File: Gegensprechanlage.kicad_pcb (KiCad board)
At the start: 2 copper layers, 42.4 x 27.8 mm, 13 parts, among them J1 To other, P1 22k, SW1 SW_Push, U1 LM386

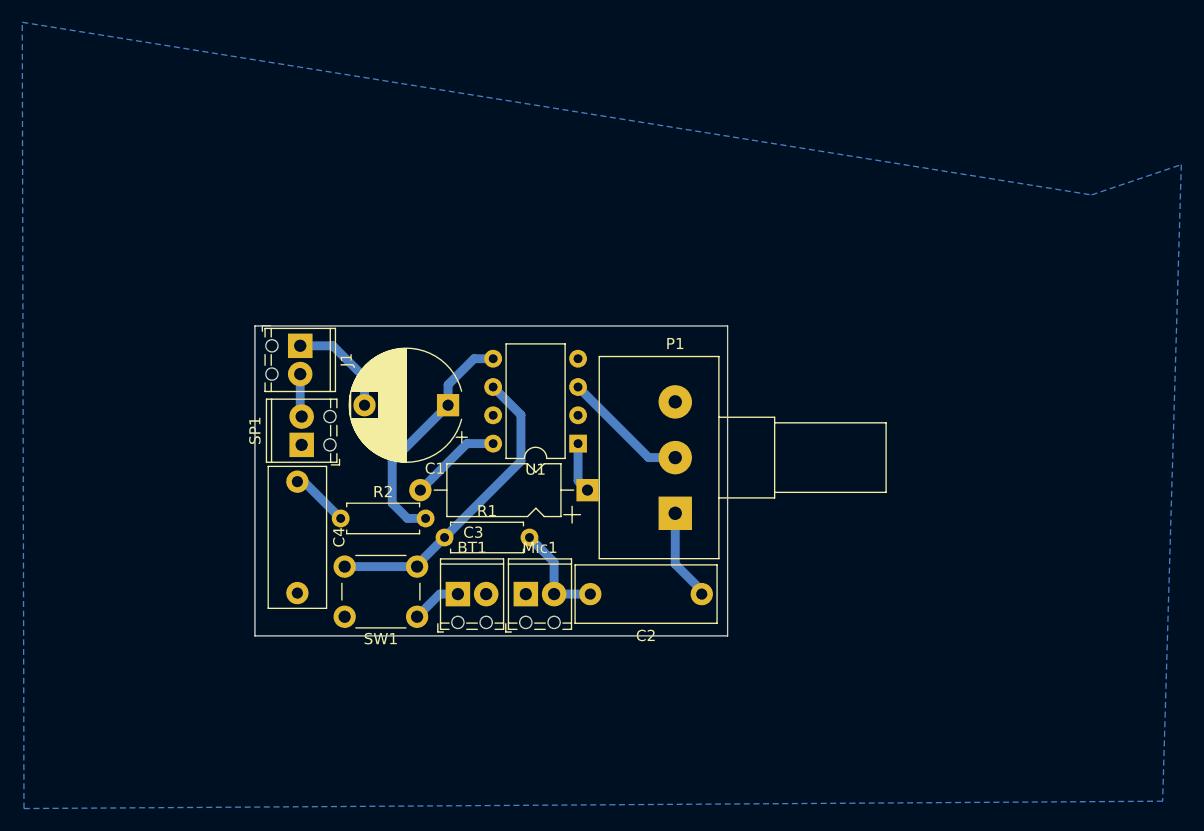
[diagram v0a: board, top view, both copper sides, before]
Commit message: Prepare for milling v1.0
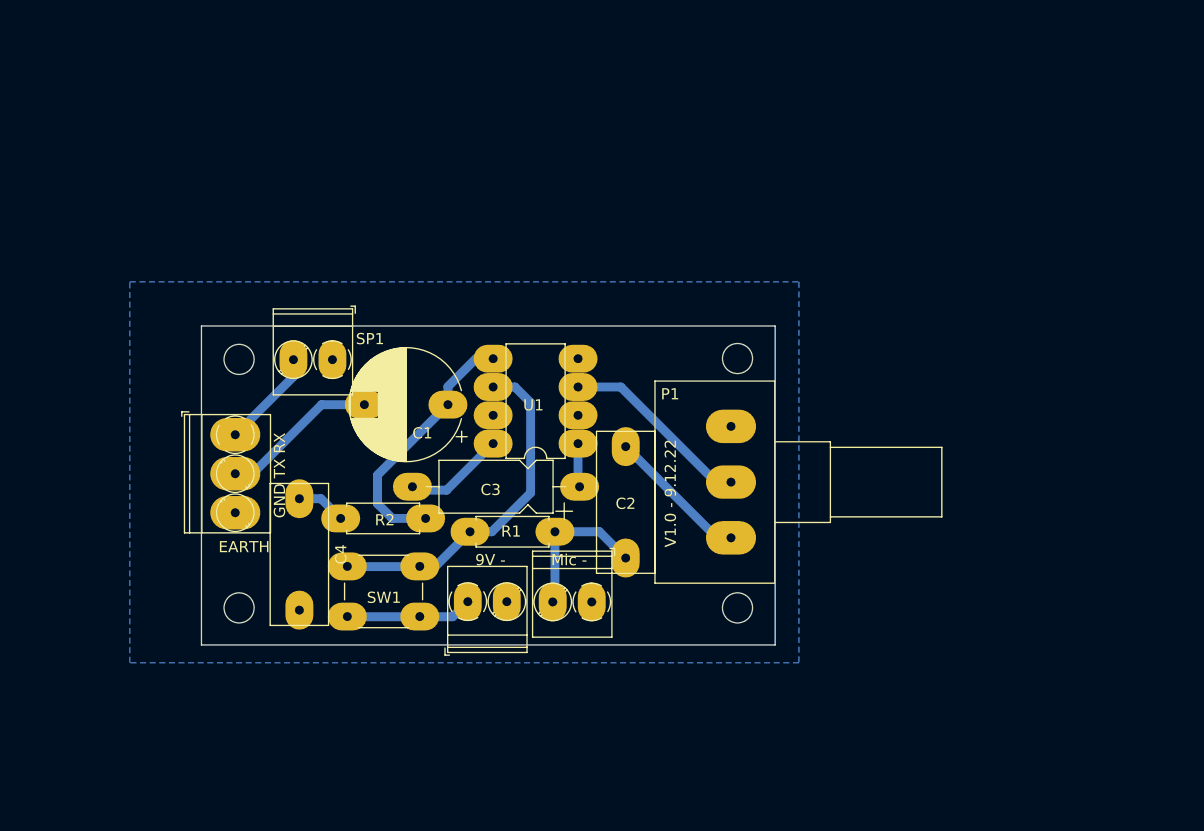
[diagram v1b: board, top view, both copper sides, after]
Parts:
- added H1: MountingHole, MountingHole:MountingHole_2.7mm_M2.5, F.Cu at (127.5, 79.4)
- added H2: MountingHole, MountingHole:MountingHole_2.7mm_M2.5, F.Cu at (82.8, 101.8)
- added H3: MountingHole, MountingHole:MountingHole_2.7mm_M2.5, F.Cu at (82.8, 79.5)
- added H4: MountingHole, MountingHole:MountingHole_2.7mm_M2.5, F.Cu at (127.5, 101.8)
- 9V -: renamed from BT1; footprint TerminalBlock_Phoenix:TerminalBlock_Phoenix_MPT-0,5-2-2.54_1x02_P2.54mm_Horizontal -> TerminalBlock_Phoenix:TerminalBlock_Phoenix_PT-1,5-2-3.5-H_1x02_P3.50mm_Horizontal
- GND TX RX: renamed from J1; footprint TerminalBlock_Phoenix:TerminalBlock_Phoenix_MPT-0,5-2-2.54_1x02_P2.54mm_Horizontal -> TerminalBlock_Phoenix:TerminalBlock_Phoenix_PT-1,5-3-3.5-H_1x03_P3.50mm_Horizontal
- Mic -: renamed from Mic1; footprint TerminalBlock_Phoenix:TerminalBlock_Phoenix_MPT-0,5-2-2.54_1x02_P2.54mm_Horizontal -> TerminalBlock_Phoenix:TerminalBlock_Phoenix_PT-1,5-2-3.5-H_1x02_P3.50mm_Horizontal
- SP1: footprint TerminalBlock_Phoenix:TerminalBlock_Phoenix_MPT-0,5-2-2.54_1x02_P2.54mm_Horizontal -> TerminalBlock_Phoenix:TerminalBlock_Phoenix_PT-1,5-2-3.5-H_1x02_P3.50mm_Horizontal
- moved C2 14.9 mm to (117.5, 87.3), turned to -90 degrees
- moved GND TX RX 9.88 mm to (82.4, 86.2)
- moved SP1 8.13 mm to (91.2, 79.5), turned to 180 degrees
- moved Mic - 5.96 mm to (114.4, 101.2), turned to 180 degrees
- moved P1 5.47 mm to (126.9, 95.5)
- moved R1 2.34 mm to (103.5, 94.9)
- moved C4 1.54 mm to (88.2, 92.0)
- moved 9V - 1.12 mm to (103.3, 101.2)
- moved C3 0.77 mm to (113.3, 90.9)
- moved SW1 0.24 mm to (99.0, 102.5)
- moved C1 0.05 mm to (101.5, 83.5)
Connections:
- GND TX RX pad 1: Net-(C1-Pad2) -> Net-(J1-Pad1)
- GND TX RX pad 2: Net-(J1-Pad2) -> Net-(C1-Pad2)
- SP1 pad 2: Net-(J1-Pad2) -> Net-(J1-Pad1)
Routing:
- net Net-(J1-Pad1): track 0.00 -> 8.95 mm
- net Net-(BT1-Pad1): track 4.50 -> 11.6 mm
- net Net-(P1-Pad2): track 11.3 -> 17.3 mm
- net Net-(C1-Pad2): track 9.44 -> 14.2 mm
- net Net-(C2-Pad1): track 8.36 -> 12.8 mm
- net Net-(C2-Pad2): track 9.55 -> 13.8 mm
- net Net-(R1-Pad1): track 27.5 -> 31.5 mm
- net Net-(J1-Pad2): track 3.86 -> 0.00 mm
- net Net-(C1-Pad1): track 21.3 -> 23.1 mm
- net Net-(C4-Pad1): track 5.25 -> 4.19 mm
- net Net-(C3-Pad2): track 8.26 -> 8.97 mm
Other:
- board size 42.4 x 27.8 mm -> 51.5 x 28.6 mm
- board text added: "EARTH"
- board text added: "V1.0 - 9.12.22"
- board text removed: "V1.0 - 8.12.22"
